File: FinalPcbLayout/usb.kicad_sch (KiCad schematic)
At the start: 26 parts, among them J5 USB_C_Receptacle, Q2 S8050, Q3 S8050, U6 FT232HPQ, U7 93LCxxB, Y1 12Mhz

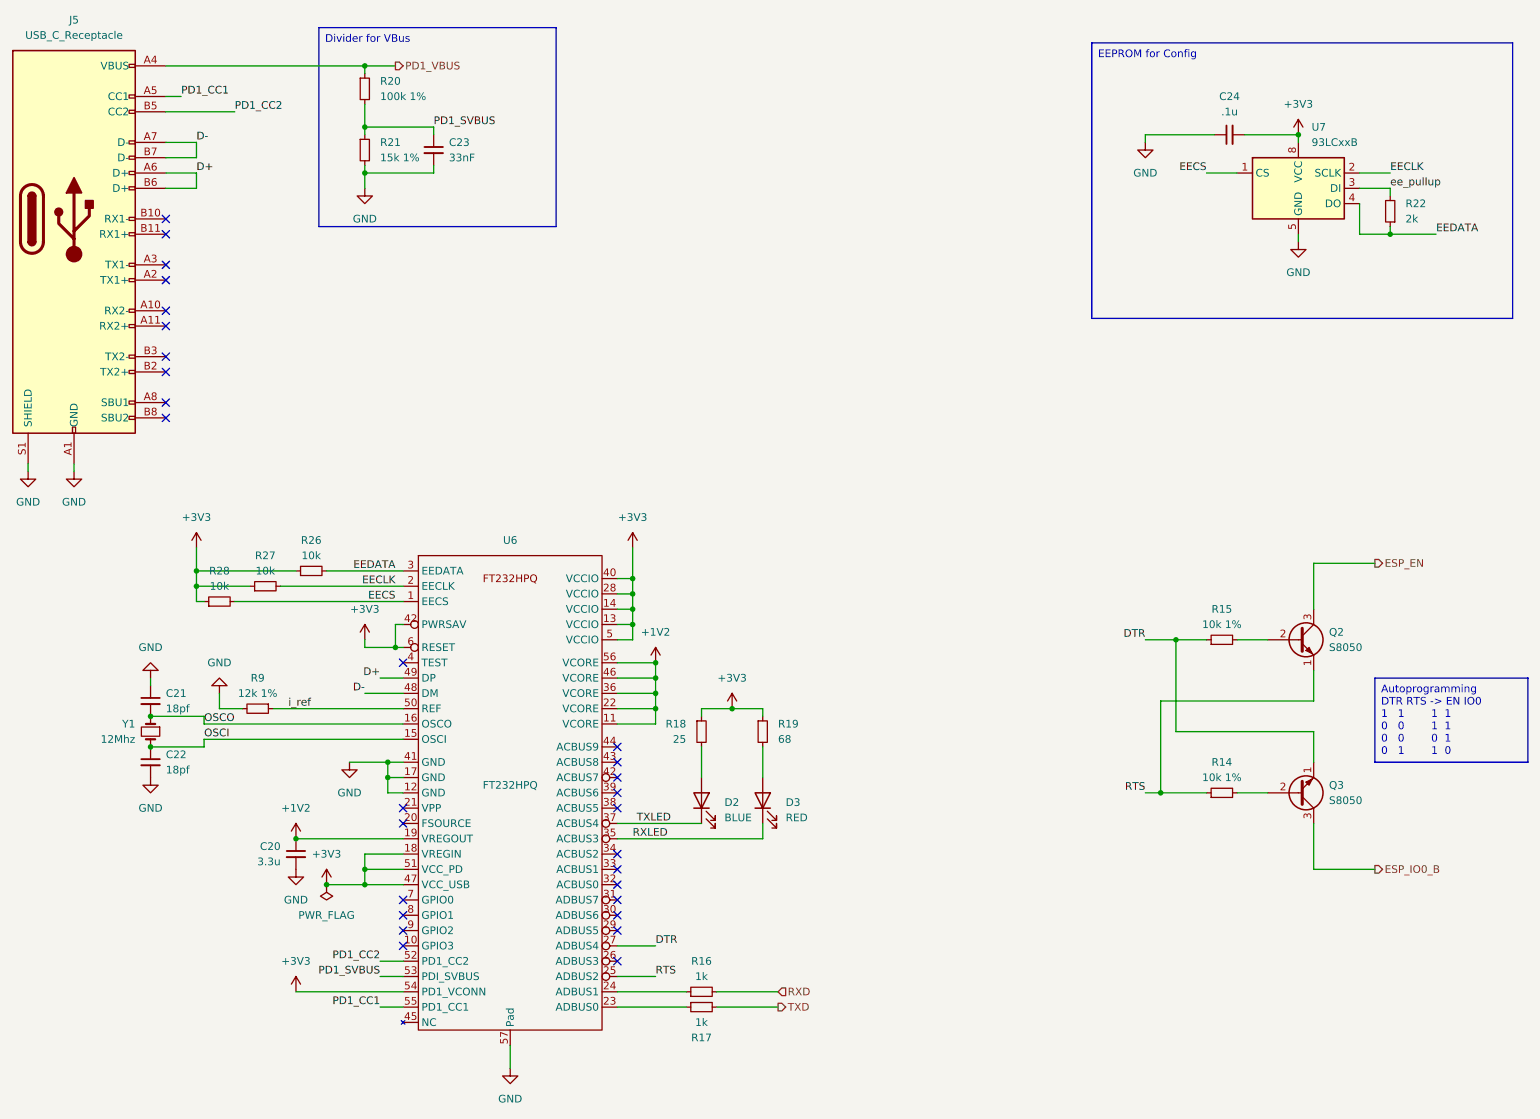
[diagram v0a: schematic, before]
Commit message: Updated CSV
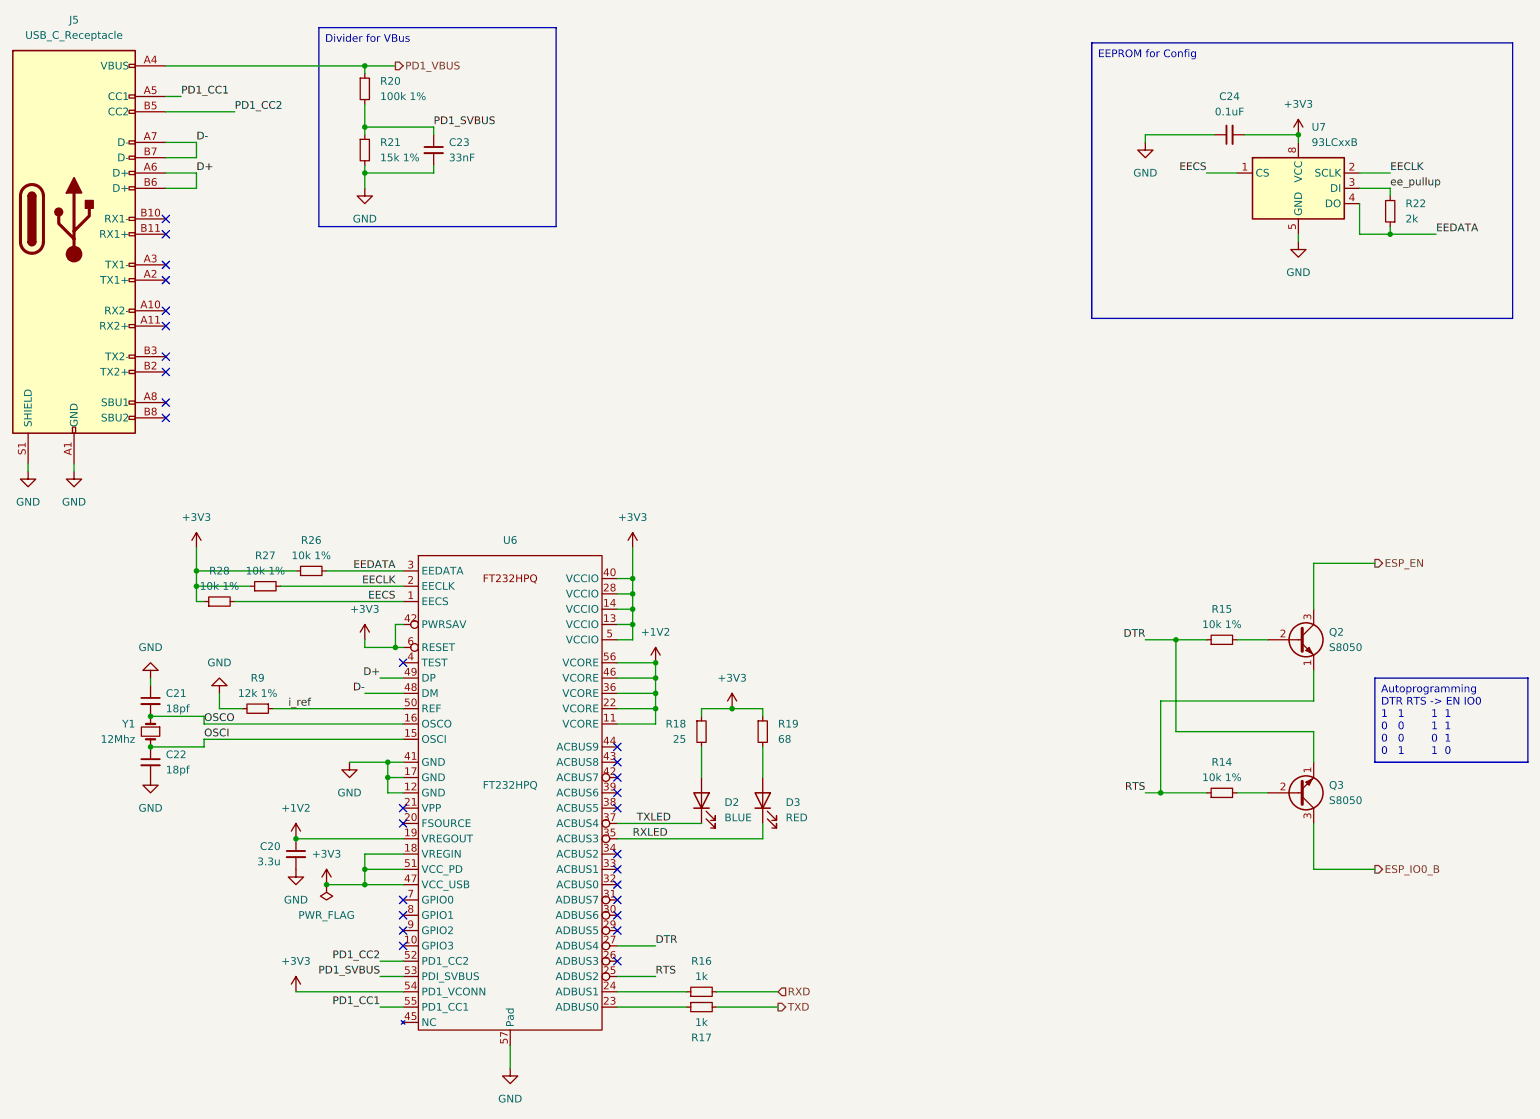
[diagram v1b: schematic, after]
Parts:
- C20: digikey_pn (none) -> 445-7476-1-ND
- C21, C22: digikey_pn (none) -> 1292-1494-1-ND
- C23: digikey_pn (none) -> 1276-2041-1-ND
- C24: value .1u -> 0.1uF; digikey_pn (none) -> 1276-1935-1-ND
- J5: digikey_pn (none) -> WM12856CT-ND
- Q2, Q3: digikey_pn (none) -> 4878-BC547BBK-ND
- R14, R15: digikey_pn (none) -> RMCF0603FT10K0CT-ND
- R16, R17: digikey_pn (none) -> RMCF0603FT1K00CT-ND
- R18: digikey_pn (none) -> 13-RP0603BRD0725RLCT-ND
- R19: digikey_pn (none) -> 1292-WR06X680JTLCT-ND
- R20: digikey_pn (none) -> RMCF0603FT100KCT-ND
- R21: digikey_pn (none) -> P15KDBCT-ND
- R22: digikey_pn (none) -> P2.00KHCT-ND
- R26, R27, R28: value 10k -> 10k 1%; digikey_pn (none) -> RMCF0603FT10K0CT-ND
- R9: digikey_pn (none) -> RMCF0603FT12K0CT-ND
- U6: digikey_pn (none) -> 768-FT232HPQ-TRAY-ND
- Y1: digikey_pn (none) -> 3155-OSC12M-3.3I/S3TCT-ND
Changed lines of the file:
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@@
+      (effects (font (size 1.27 1.27)) hide)
+    )
+    (property "digikey_pn" "1292-1494-1-ND" (at 48.26 127 0)
       (effects (font (size 1.27 1.27)) hide)
     )
@@
       (effects (font (size 1.27 1.27)) (justify left) hide)
     )
+    (property "digikey_pn" "4878-BC547BBK-ND " (at 238.76 142.24 0)
+      (effects (font (size 1.27 1.27)) hide)
+    )
     (pin "1")
     (pin "2")
@@
       (effects (font (size 1.27 1.27)))
     )
-    (property "Value" "10k" (at 74.93 102.87 90)
+    (property "Value" "10k 1%" (at 74.93 102.87 90)
       (effects (font (size 1.27 1.27)))
     )
@@
       (effects (font (size 1.27 1.27)) hide)
     )
+    (property "digikey_pn" "RMCF0603FT10K0CT-ND" (at 74.93 105.41 0)
+      (effects (font (size 1.27 1.27)) hide)
+    )
     (pin "1")
     (pin "2")
@@
       (effects (font (size 1.27 1.27)))
     )
-    (property "Value" "10k" (at 59.69 107.95 90)
+    (property "Value" "10k 1%" (at 59.69 107.95 90)
       (effects (font (size 1.27 1.27)))
     )
@@
     )
     (property "Sim.Enable" "0" (at 59.69 110.49 0)
+      (effects (font (size 1.27 1.27)) hide)
+    )
+    (property "digikey_pn" "RMCF0603FT10K0CT-ND" (at 59.69 110.49 0)
       (effects (font (size 1.27 1.27)) hide)
     )
@@
       (effects (font (size 1.27 1.27)) (justify left) hide)
     )
+    (property "digikey_pn" "4878-BC547BBK-ND " (at 238.76 116.84 0)
+      (effects (font (size 1.27 1.27)) hide)
+    )
     (pin "1")
     (pin "2")
@@
       (effects (font (size 1.27 1.27)) hide)
     )
+    (property "digikey_pn" "1276-2041-1-ND" (at 95.25 35.56 0)
+      (effects (font (size 1.27 1.27)) hide)
+    )
     (pin "1")
     (pin "2")
@@
     )
     (property "Sim.Enable" "0" (at 48.26 137.16 0)
+      (effects (font (size 1.27 1.27)) hide)
+    )
+    (property "digikey_pn" "1292-1494-1-ND" (at 48.26 137.16 0)
       (effects (font (size 1.27 1.27)) hide)
     )
@@
       (effects (font (size 1.27 1.27)) hide)
     )
+    (property "digikey_pn" "RMCF0603FT1K00CT-ND" (at 139.7 177.8 0)
+      (effects (font (size 1.27 1.27)) hide)
+    )
     (pin "1")
     (pin "2")
@@
       (effects (font (size 1.27 1.27)) hide)
     )
+    (property "digikey_pn" "P15KDBCT-ND" (at 83.82 35.56 0)
+      (effects (font (size 1.27 1.27)) hide)
+    )
     (pin "1")
     (pin "2")
@@
       (effects (font (size 1.27 1.27)) hide)
     )
+    (property "digikey_pn" "P2.00KHCT-ND" (at 254 45.72 0)
+      (effects (font (size 1.27 1.27)) hide)
+    )
     (pin "1")
     (pin "2")
@@
     )
     (property "Sim.Enable" "0" (at 149.86 132.08 0)
+      (effects (font (size 1.27 1.27)) hide)
+    )
+    (property "digikey_pn" "1292-WR06X680JTLCT-ND " (at 149.86 132.08 0)
       (effects (font (size 1.27 1.27)) hide)
     )
@@
     )
     (property "Sim.Enable" "0" (at 139.7 132.08 0)
+      (effects (font (size 1.27 1.27)) hide)
+    )
+    (property "digikey_pn" "13-RP0603BRD0725RLCT-ND" (at 139.7 132.08 0)
       (effects (font (size 1.27 1.27)) hide)
     )
@@
       (effects (font (size 1.27 1.27)))
     )
-    (property "Value" "10k" (at 67.31 105.41 90)
+    (property "Value" "10k 1%" (at 67.31 105.41 90)
       (effects (font (size 1.27 1.27)))
     )
@@
     )
     (property "Sim.Enable" "0" (at 67.31 107.95 0)
+      (effects (font (size 1.27 1.27)) hide)
+    )
+    (property "digikey_pn" "RMCF0603FT10K0CT-ND" (at 67.31 107.95 0)
       (effects (font (size 1.27 1.27)) hide)
     )
@@
       (effects (font (size 1.27 1.27)) hide)
     )
+    (property "digikey_pn" "445-7476-1-ND" (at 72.39 152.4 0)
+      (effects (font (size 1.27 1.27)) hide)
+    )
     (pin "1")
     (pin "2")
@@
       (effects (font (size 1.27 1.27)) hide)
     )
+    (property "digikey_pn" "RMCF0603FT10K0CT-ND" (at 226.06 116.84 0)
+      (effects (font (size 1.27 1.27)) hide)
+    )
     (pin "1")
     (pin "2")
@@
     )
     (property "Sim.Enable" "0" (at 226.06 142.24 0)
+      (effects (font (size 1.27 1.27)) hide)
+    )
+    (property "digikey_pn" "RMCF0603FT10K0CT-ND" (at 226.06 142.24 0)
       (effects (font (size 1.27 1.27)) hide)
     )
@@
     )
     (property "Sim.Enable" "0" (at 107.95 142.24 0)
+      (effects (font (size 1.27 1.27)) hide)
+    )
+    (property "digikey_pn" "768-FT232HPQ-TRAY-ND " (at 107.95 142.24 0)
       (effects (font (size 1.27 1.27)) hide)
     )
@@
       (effects (font (size 1.27 1.27)) hide)
     )
+    (property "digikey_pn" "3155-OSC12M-3.3I/S3TCT-ND" (at 48.26 132.08 0)
+      (effects (font (size 1.27 1.27)) hide)
+    )
     (pin "1")
     (pin "2")
@@
     )
     (property "Sim.Enable" "0" (at 35.56 46.99 0)
+      (effects (font (size 1.27 1.27)) hide)
+    )
+    (property "digikey_pn" "WM12856CT-ND" (at 35.56 46.99 0)
       (effects (font (size 1.27 1.27)) hide)
     )
@@
       (effects (font (size 1.27 1.27)) hide)
     )
+    (property "digikey_pn" "RMCF0603FT1K00CT-ND" (at 139.7 175.26 0)
+      (effects (font (size 1.27 1.27)) hide)
+    )
     (pin "1")
     (pin "2")
@@
       (effects (font (size 1.27 1.27)) hide)
     )
+    (property "digikey_pn" "RMCF0603FT100KCT-ND" (at 83.82 25.4 0)
+      (effects (font (size 1.27 1.27)) hide)
+    )
     (pin "1")
     (pin "2")
@@
       (effects (font (size 1.27 1.27)))
     )
-    (property "Value" ".1u" (at 227.3363 29.21 90)
+    (property "Value" "0.1uF" (at 227.3363 29.21 90)
       (effects (font (size 1.27 1.27)))
     )
@@
       (effects (font (size 1.27 1.27)) hide)
     )
+    (property "digikey_pn" "1276-1935-1-ND" (at 227.33 33.02 0)
+      (effects (font (size 1.27 1.27)) hide)
+    )
     (pin "1")
     (pin "2")
@@
       (effects (font (size 1.27 1.27)) hide)
     )
+    (property "digikey_pn" "RMCF0603FT12K0CT-ND" (at 66.04 128.27 0)
+      (effects (font (size 1.27 1.27)) hide)
+    )
